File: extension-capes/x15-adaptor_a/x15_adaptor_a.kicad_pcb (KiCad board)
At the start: 2 copper layers, 39 x 46 mm, 67 parts, among them P1 FX18-60S-0.8SV15, P2 I2S, P3 SPI

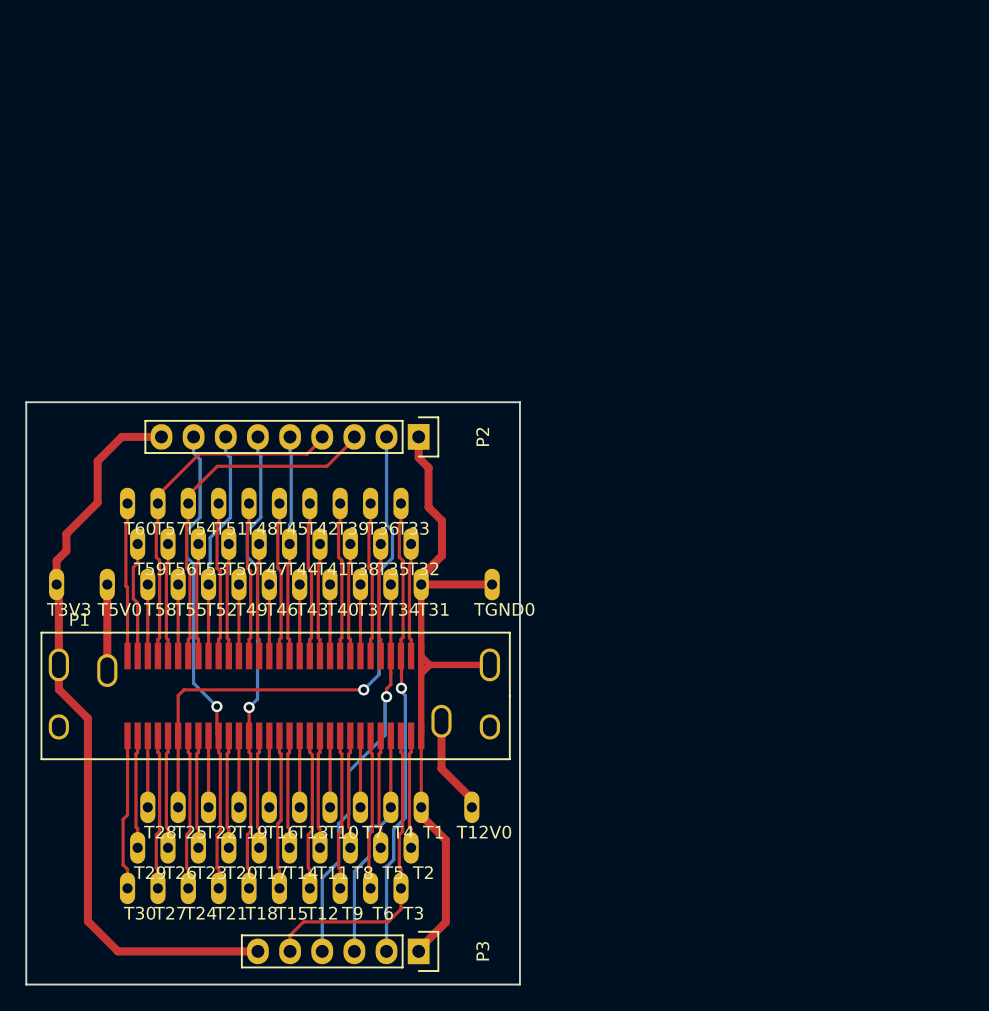
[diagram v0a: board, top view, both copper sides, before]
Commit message: x15 adaptor production stage
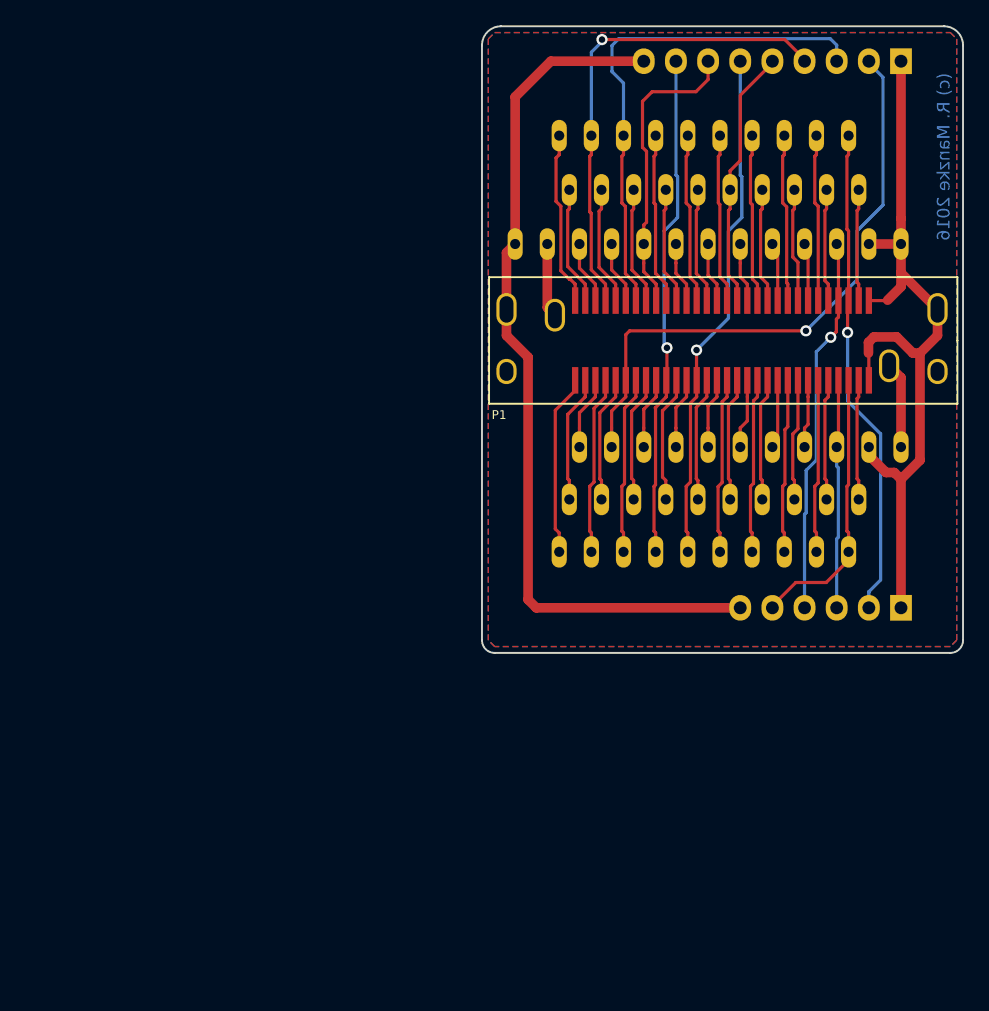
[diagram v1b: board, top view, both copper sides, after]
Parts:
- added G***: LOGO, modules:cc-logo, B.Cu at (142.2, 92.5)
- P2, P3, T1, T10, T11, T12, T12V0, T13, T14, T15, T16, T17, T18, T19, T2, T20, T21, T22, T23, T24, T25, T26, T27, T28, T29, T3, T30, T31, T32, T33, T34, T35, T36, T37, T38, T39, T3V3, T4, T40, T41, T42, T43, T44, T45, T46, T47, T48, T49, T5, T50, T51, T52, T53, T54, T55, T56, T57, T58, T59, T5V0, T6, T60, T7, T8, T9, TGND0: moved to B.Cu
- moved P2 48.3 mm to (165.5, 49.1), turned to 90 degrees
- moved P3 46.8 mm to (165.5, 92.2), turned to 90 degrees
- moved T33 45.8 mm to (161.4, 54.9)
- moved T36 45.7 mm to (158.8, 54.9)
- moved T39 45.6 mm to (156.3, 54.9)
- moved T42 45.4 mm to (153.7, 54.9)
- moved T1 45.4 mm to (163.0, 79.5)
- moved T45 45.3 mm to (151.2, 54.9)
- moved T4 45.3 mm to (160.4, 79.5)
- moved T48 45.2 mm to (148.7, 54.9)
- moved T7 45.2 mm to (157.9, 79.5)
- moved P1 45.2 mm to (163.0, 71.1)
- moved T51 45.1 mm to (146.1, 54.9)
- moved T3V3 45.1 mm to (135.0, 63.5)
- moved T32 45.1 mm to (162.2, 59.2)
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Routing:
- net /ASDATA1: track 28.0 -> 40.5 mm
- net /ALRCLK: track 27.9 -> 38.3 mm, vias 0 -> 1
- net /3V3: track 59.2 -> 69.1 mm
- net GND: track 56.3 -> 64.0 mm
- net /DLRCLK: track 18.2 -> 23.7 mm
- net /DSDATA1: track 37.0 -> 40.7 mm
- net /RESET: track 44.8 -> 48.0 mm
- net /ABCLK: track 17.5 -> 20.6 mm
- net /SPI_CS: track 24.8 -> 22.0 mm
- net /SPI_DO: track 36.4 -> 38.9 mm
- net /DBCLK: track 37.6 -> 39.8 mm
- net Net-(P1-Pad27): track 12.3 -> 14.1 mm
- net Net-(P1-Pad24): track 12.3 -> 14.1 mm
- net Net-(P1-Pad60): track 12.2 -> 13.8 mm
- net Net-(P1-Pad15): track 12.3 -> 13.9 mm
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- added copper zone on B.Cu, net GND
- added copper zone on F.Cu, net GND
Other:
- board size 39 x 46 mm -> 38 x 49.5 mm
- rule pad_to_mask_clearance: 0.2 -> 0.0381
- board text added: "(c) R. Manzke 2016"
- board text added: "CTAG X15 Breakout Brd. Rev. A www.creative-technologies.de"
